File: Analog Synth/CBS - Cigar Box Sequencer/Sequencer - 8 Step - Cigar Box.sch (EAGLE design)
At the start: 187 parts, among them IC1 TL084P, IC10 79L05, IC11 MCP6002, IC12 74AC138N, IC13 74ALS04N, IC14 74AC138N, IC15 74ALS04N, IC16 74ALS04N, IC2 TL084P, IC3 TL084P, IC4 74ALS04N, IC5 4050N, IC6 78L05, IC7 40193N, IC8 78L05, IC9 74LS86N, Q1 I/O, Q14 J310, Q15 J310, Q16 J310, Q17 J310, Q18 J310, Q19 J310, Q2 I/O, Q20 J310, Q3 I/O, Q4 2N3906, Q5 2N3904, Q6 J310, X1 I/O, X2 I/O, X3 I/O

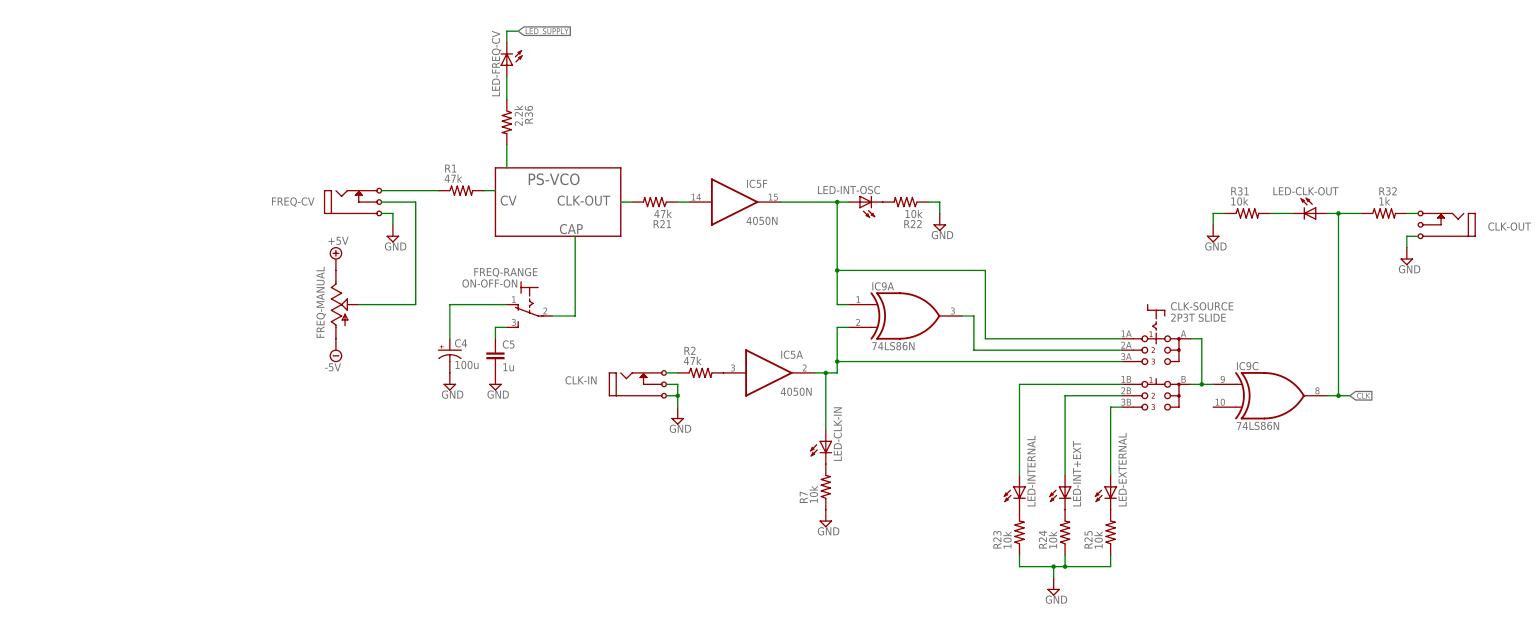
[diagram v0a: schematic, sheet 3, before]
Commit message: CBS: schematic (stillstill)
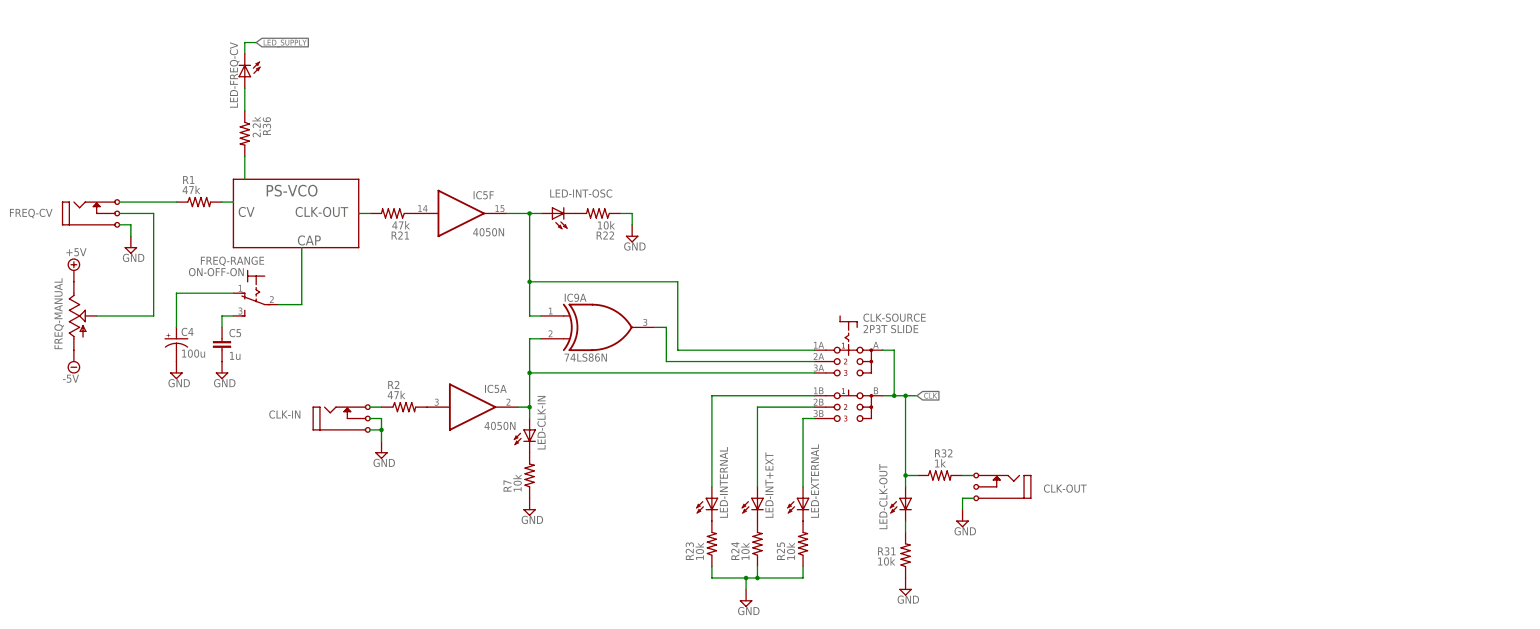
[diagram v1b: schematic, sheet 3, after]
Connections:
- net CLK: no longer IC9C.O
- net N$46: no longer IC9C.I0
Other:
- moved on the sheet: C4, C5, CLK-IN, CLK-OUT, CLK-SOURCE, FREQ-CV, FREQ-MANUAL, FREQ-RANGE, IC5A, IC5F, IC9A, LED-CLK-IN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
